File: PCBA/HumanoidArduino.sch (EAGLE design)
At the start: 46 parts, among them IC1 7805TV, J2 22-27-2041-04

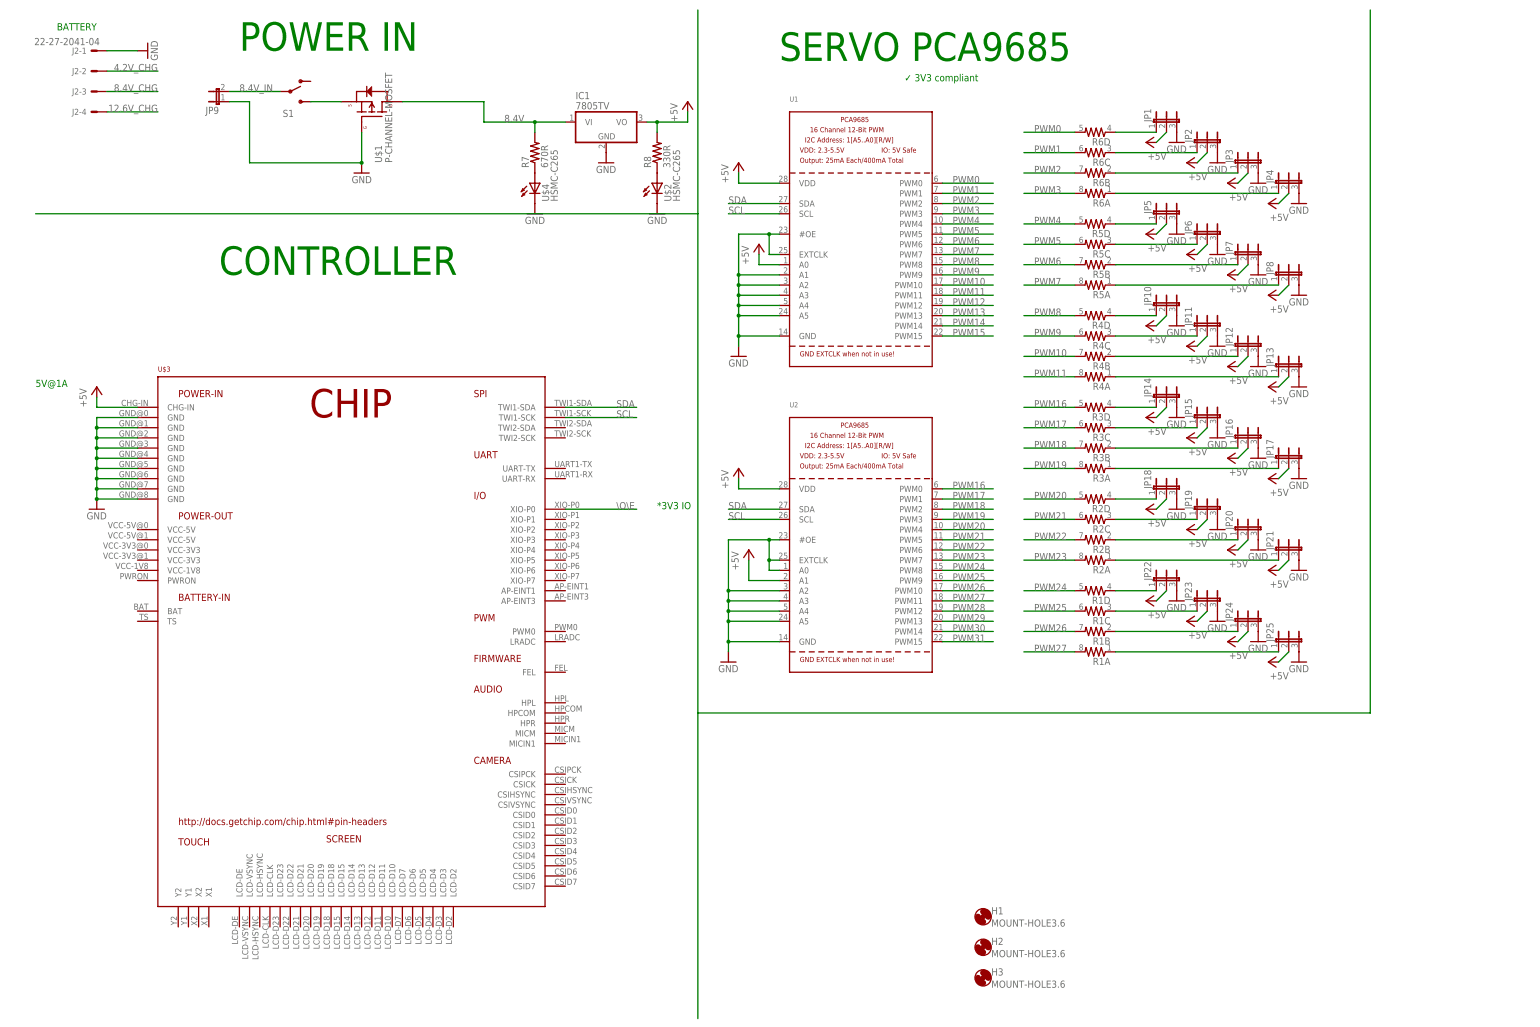
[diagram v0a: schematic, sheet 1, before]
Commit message: more PCBA work
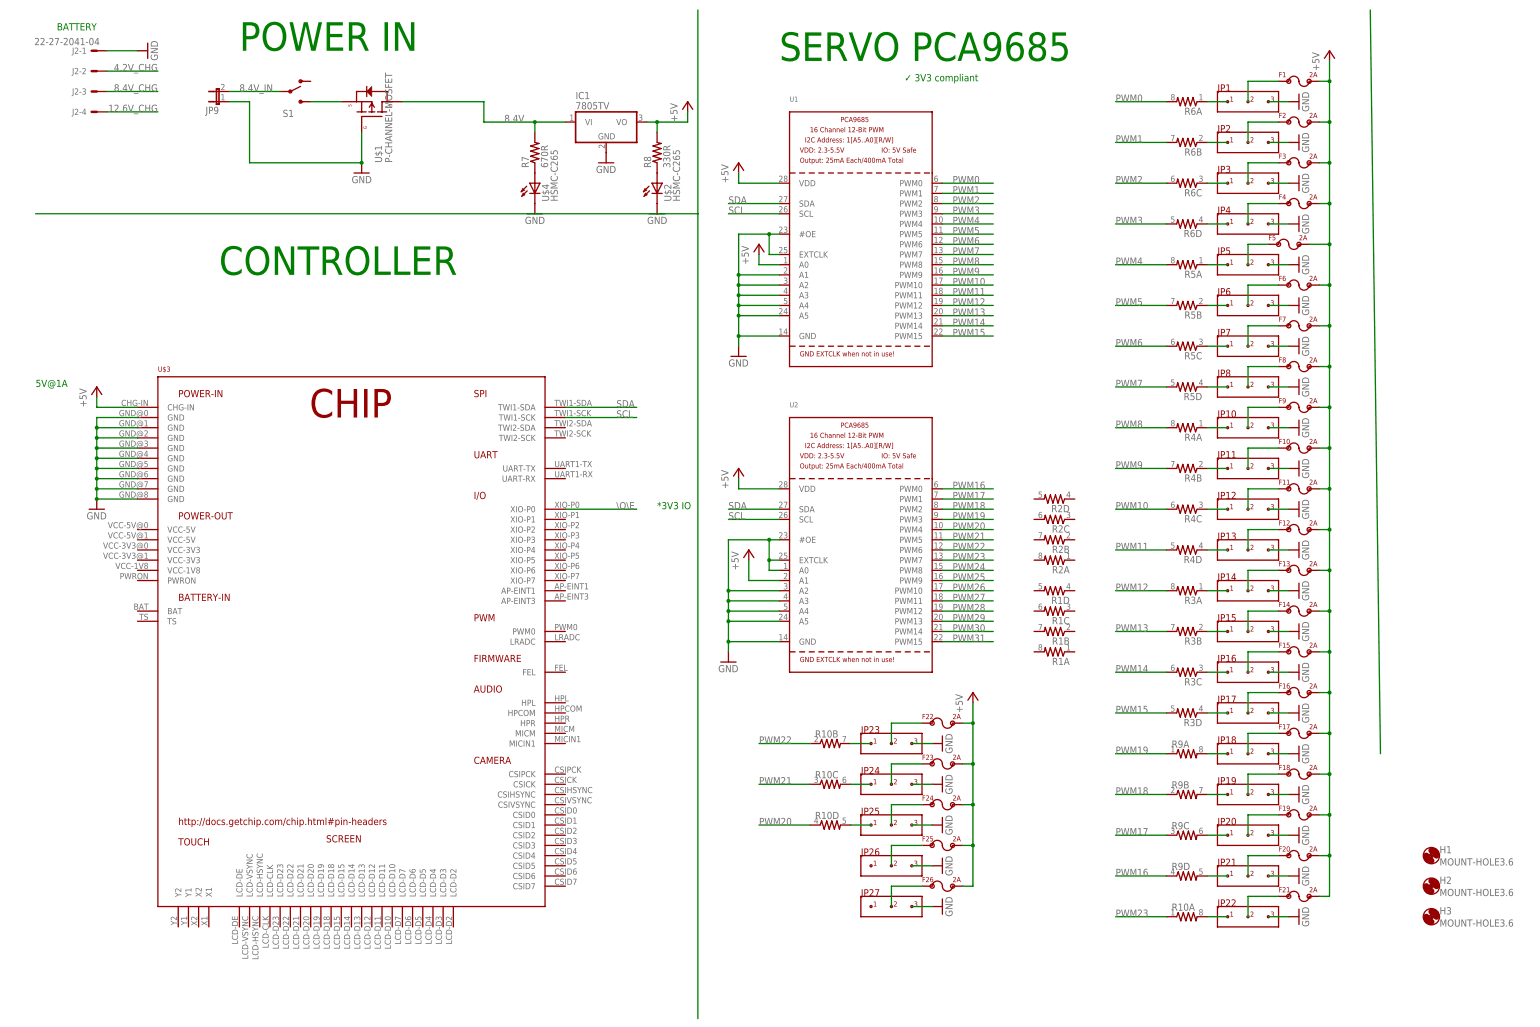
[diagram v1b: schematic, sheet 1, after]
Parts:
- added F1, F10, F11, F12, F13, F14, F15, F16, F17, F18, F19, F2, F20, F21, F22, F23, F24, F25, F26, F3, F4, F5, F6, F7, F8, F9: POLYSWITCH, HumanoidLbr:POLYSWITCH
- added JP26, JP27: JUMPER_3X1_0.1, HumanoidLbr:JUMPER_3X1_0.1
- added R10, R9: (no value), SparkFun-Resistors:RESISTOR-ARRAY0603-ARV
- JP1, JP10, JP11, JP12, JP13, JP14, JP15, JP16, JP17, JP18, JP19, JP2, JP20, JP21, JP22, JP23, JP24, JP25, JP3, JP4, JP5, JP6, JP7, JP8: value (none) -> JUMPER_3X1_0.1; device jumper:JP2E -> HumanoidLbr:JUMPER_3X1_0.1
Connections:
- removed net +5V1: JP10.2, JP11.2, JP12.2, JP13.2, JP14.2, JP15.2, JP16.2, JP17.2, JP18.2, JP19.2, JP20.2, JP21.2, JP22.2, JP23.2, JP24.2, JP25.2
- new net N$27: F1.P$1, JP1.2
- new net N$30: F2.P$1, JP2.2
- new net N$31: JP12.1, R4C.1
- new net N$32: JP13.1, R4D.1
- new net N$33: JP14.1, R3A.1
- new net N$34: JP15.1, R3B.1
- new net N$35: JP16.1, R3C.1
- new net N$36: JP17.1, R3D.1
- new net N$38: F21.P$1, JP22.2
- new net N$39: F20.P$1, JP21.2
- new net N$40: F19.P$1, JP20.2
- new net N$41: F18.P$1, JP19.2
- new net N$42: F17.P$1, JP18.2
- new net N$43: JP18.1, R9A.2
- new net N$44: JP19.1, R9B.2
- new net N$45: JP20.1, R9C.2
- new net N$46: JP21.1, R9D.2
- new net N$47: JP22.1, R10A.2
- new net N$48: F22.P$1, JP23.2
- new net N$49: F23.P$1, JP24.2
- new net N$50: F24.P$1, JP25.2
- new net N$51: F25.P$1, JP26.2
- new net N$52: F26.P$1, JP27.2
- new net N$53: JP23.1, R10B.2
- new net N$54: JP24.1, R10C.2
- new net N$55: JP25.1, R10D.2
- net +5V: now also F1.P$2, F10.P$2, F11.P$2, F12.P$2, F13.P$2, F14.P$2, F15.P$2, F16.P$2, F17.P$2, F18.P$2, F19.P$2, F2.P$2, F20.P$2, F21.P$2, F22.P$2, F23.P$2, F24.P$2, F25.P$2, F26.P$2, F3.P$2, F4.P$2, F5.P$2, F6.P$2, F7.P$2, F8.P$2, F9.P$2; no longer JP1.2, JP2.2, JP3.2, JP4.2, JP5.2, JP6.2, JP7.2, JP8.2
- net GND: now also JP26.3, JP27.3; no longer JP10.3, JP11.3, JP12.3, JP13.3, JP14.3, JP15.3, JP16.3, JP17.3, JP5.3, JP6.3, JP7.3, JP8.3
- net N$10: now also F14.P$1, JP15.2; no longer JP10.1, R4D.1
- net N$11: now also F13.P$1, JP14.2; no longer JP11.1, R4C.1
- net N$12: now also F12.P$1, JP13.2; no longer JP12.1, R4B.1
- net N$13: now also F11.P$1, JP12.2; no longer JP13.1, R4A.1
- net N$14: now also F10.P$1, JP11.2; no longer JP14.1, R3D.1
- net N$15: now also F9.P$1, JP10.2; no longer JP15.1, R3C.1
- net N$16: now also F8.P$1, JP8.2; no longer JP16.1, R3B.1
- net N$17: now also F7.P$1, JP7.2; no longer JP17.1, R3A.1
- net N$18: now also F6.P$1, JP6.2; no longer JP18.1, R2D.1
- net N$19: now also F5.P$1, JP5.2; no longer JP19.1, R2C.1
- net N$2: now also R6A.1; no longer R6D.1
- net N$20: now also JP5.1, R5A.1; no longer JP20.1, R2B.1
- net N$21: now also JP6.1, R5B.1; no longer JP21.1, R2A.1
- net N$22: now also JP7.1, R5C.1; no longer JP22.1, R1D.1
- net N$23: now also JP8.1, R5D.1; no longer JP23.1, R1C.1
- net N$24: now also JP10.1, R4A.1; no longer JP24.1, R1B.1
- net N$25: now also JP11.1, R4B.1; no longer JP25.1, R1A.1
- net N$3: now also R6B.1; no longer R6C.1
- net N$4: now also R6C.1; no longer R6B.1
- net N$5: now also R6D.1; no longer R6A.1
- net N$6: now also F3.P$1, JP3.2; no longer JP5.1, R5D.1
- net N$7: now also F4.P$1, JP4.2; no longer JP6.1, R5C.1
- net N$8: now also F16.P$1, JP17.2; no longer JP7.1, R5B.1
- net N$9: now also F15.P$1, JP16.2; no longer JP8.1, R5A.1
- net PWM0: now also R6A.2; no longer R6D.2
- net PWM1: now also R6B.2; no longer R6C.2
- net PWM10: now also R4C.2; no longer R4B.2
- net PWM11: now also R4D.2; no longer R4A.2
- net PWM12: now also R3A.2
- net PWM13: now also R3B.2
- net PWM14: now also R3C.2
- net PWM15: now also R3D.2
- net PWM16: now also R9D.1; no longer R3D.2
- net PWM17: now also R9C.1; no longer R3C.2
- net PWM18: now also R9B.1; no longer R3B.2
- net PWM19: now also R9A.1; no longer R3A.2
- net PWM2: now also R6C.2; no longer R6B.2
- net PWM20: now also R10D.1; no longer R2D.2
- net PWM21: now also R10C.1; no longer R2C.2
- net PWM22: no longer R2B.2
- net PWM23: now also R10A.1; no longer R2A.2
- net PWM24: no longer R1D.2
- net PWM25: no longer R1C.2
- net PWM26: no longer R1B.2
- net PWM27: no longer R1A.2
- net PWM3: now also R6D.2; no longer R6A.2
- net PWM4: now also R5A.2; no longer R5D.2
- net PWM5: now also R5B.2; no longer R5C.2
- net PWM6: now also R5C.2; no longer R5B.2
- net PWM7: now also R5D.2; no longer R5A.2
- net PWM8: now also R4A.2; no longer R4D.2
- net PWM9: now also R4B.2; no longer R4C.2
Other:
- moved on the sheet: H1, H2, H3, R1A, R1B, R1C, R1D, R2A, R2B, R2C, R2D, R3A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
